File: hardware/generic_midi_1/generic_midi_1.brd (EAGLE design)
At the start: 47.3 x 44.1 mm, 26 parts, among them IC1 MEGA168/328, IC2 RFM12

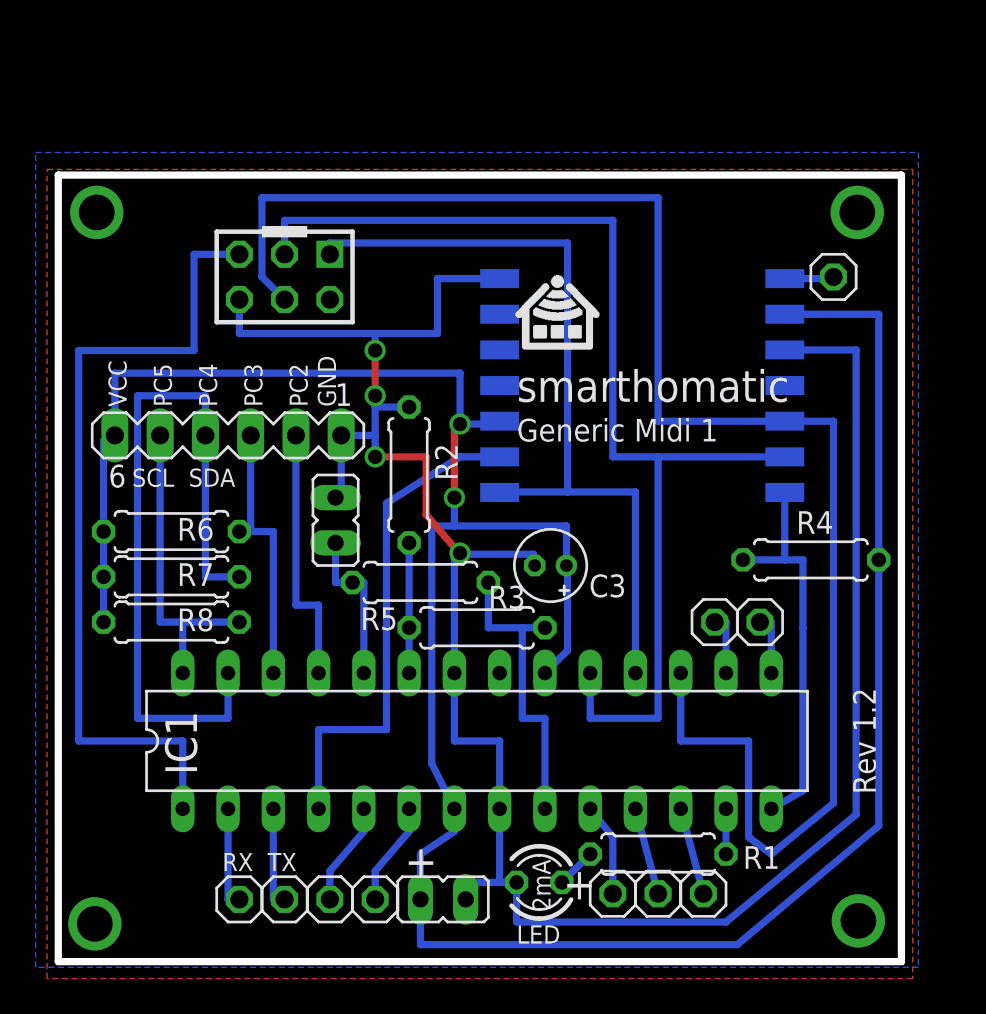
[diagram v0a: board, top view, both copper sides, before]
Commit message: test
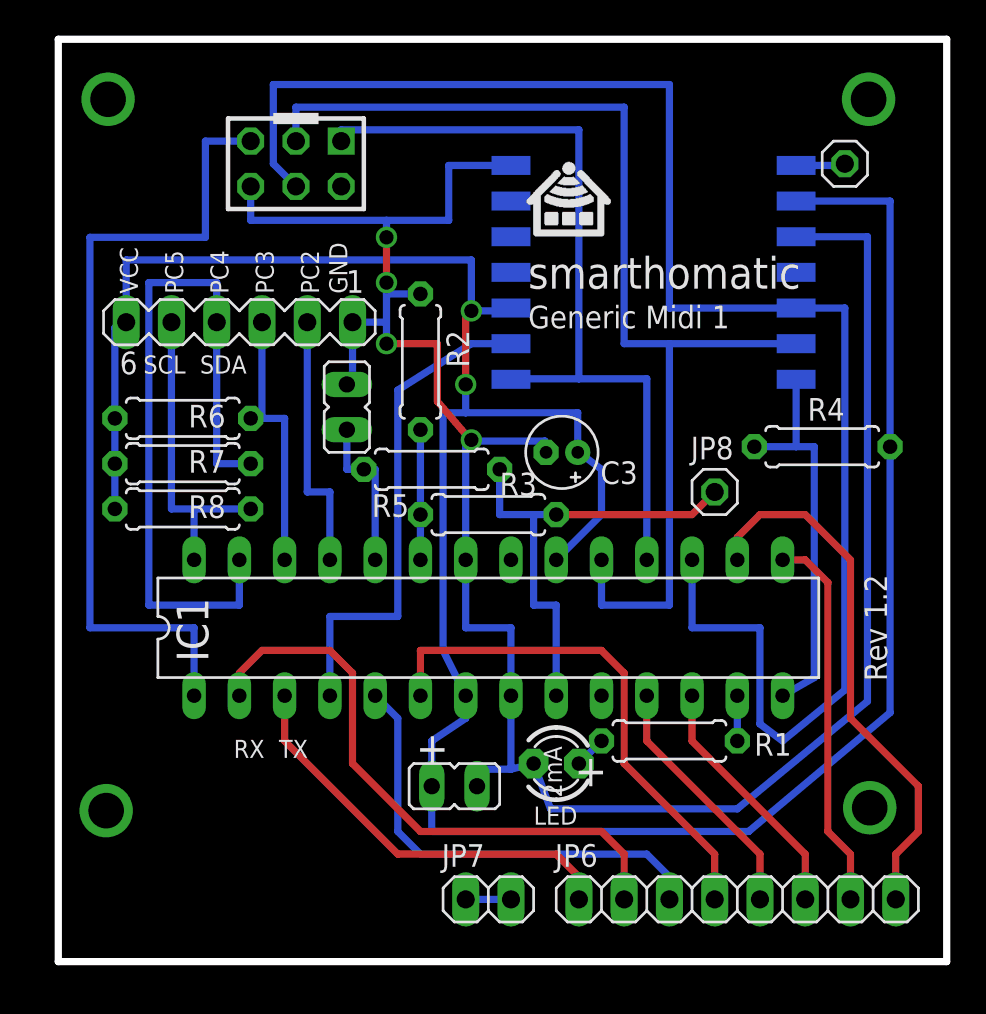
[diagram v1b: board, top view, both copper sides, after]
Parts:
- removed JP10: PD6, pinhead:1X01
- removed JP11: PD4, pinhead:1X01
- removed JP12: PD3, pinhead:1X01
- removed JP13: PB7, pinhead:1X01
- removed JP14: PD0, pinhead:1X01
- removed JP9: PD5, pinhead:1X01
- JP6: value PB1 -> (none); device pinhead:1X01 -> pinhead:1X08
- JP7: value PB2 -> (none); device pinhead:1X01 -> pinhead:1X02
- JP8: value PD1 -> (none)
- moved JP8 33.2 mm to (36.8, 26.7)
- moved JP7 20.1 mm to (24.1, 3.81)
- moved JP6 15.6 mm to (38.1, 3.81)
- moved LED 6.74 mm to (27.9, 11.4)
- moved IC1 6.38 mm to (24.1, 19.1)
- moved IC2 6.38 mm to (25.4, 47.0)
- moved JP1 6.38 mm to (13.3, 45.1)
- moved JP2 6.38 mm to (10.2, 36.2)
- moved JP3 6.38 mm to (16.2, 31.4)
- moved JP5 6.38 mm to (44.1, 45.1)
- moved R4 6.38 mm to (42.9, 29.2)
- moved R5 6.38 mm to (21.0, 27.9)
- moved R7 6.38 mm to (6.99, 28.3)
- moved R8 6.38 mm to (6.99, 25.7)
- moved JP4 6.38 mm to (22.2, 10.2)
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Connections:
- removed net N$16: IC1.12, JP10.1
- removed net N$17: IC1.15, JP6.1
- removed net N$19: IC1.16, JP7.1
- removed net N$20: IC1.3, JP8.1
- removed net N$22: IC1.6, JP11.1
- removed net N$23: IC1.5, JP12.1
- removed net N$25: IC1.10, JP13.1
- removed net N$26: IC1.2, JP14.1
- new net IO0: IC1.3, JP6.1
- new net IO1: IC1.2, JP6.2
- new net IO2: IC1.5, JP6.3
- new net IO3: IC1.6, JP6.4
- new net IO4: IC1.11, JP6.5
- new net IO5: IC1.12, JP6.6
- new net IO6: IC1.15, JP6.7
- new net IO7: IC1.16, JP6.8
- net N$14: now also IC1.10, JP7.1, JP7.2; no longer IC1.11, JP9.1
- net N$24: now also JP8.1
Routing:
- net IO1: track 0.00 -> 33.6 mm
- net IO7: track 0.00 -> 30.4 mm
- net IO3: track 0.00 -> 29.3 mm
- net IO2: track 0.00 -> 25.7 mm
- net IO0: track 0.00 -> 23.5 mm
- net IO6: track 0.00 -> 21.4 mm
- net IO5: track 0.00 -> 14.1 mm
- net IO4: track 0.00 -> 14.1 mm
- net N$24: track 17.1 -> 26.6 mm
- net N$23: track 5.78 -> 0.00 mm
- net N$22: track 5.78 -> 0.00 mm
- net N$26: track 5.71 -> 0.00 mm
- net N$20: track 5.71 -> 0.00 mm
- net N$25: track 5.21 -> 0.00 mm
- net N$16: track 4.93 -> 0.00 mm
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- removed copper zone on layer 1, net GND
- removed copper zone on layer 16, net GND
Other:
- board size 47.3 x 44.1 mm -> 49.8 x 51.8 mm
